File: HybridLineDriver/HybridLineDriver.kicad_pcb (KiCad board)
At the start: 2 copper layers, 100 x 100 mm, 34 parts, among them J1 XLR3, J2 Conn_01x03, J3 Conn_01x02, U1 OPA1679

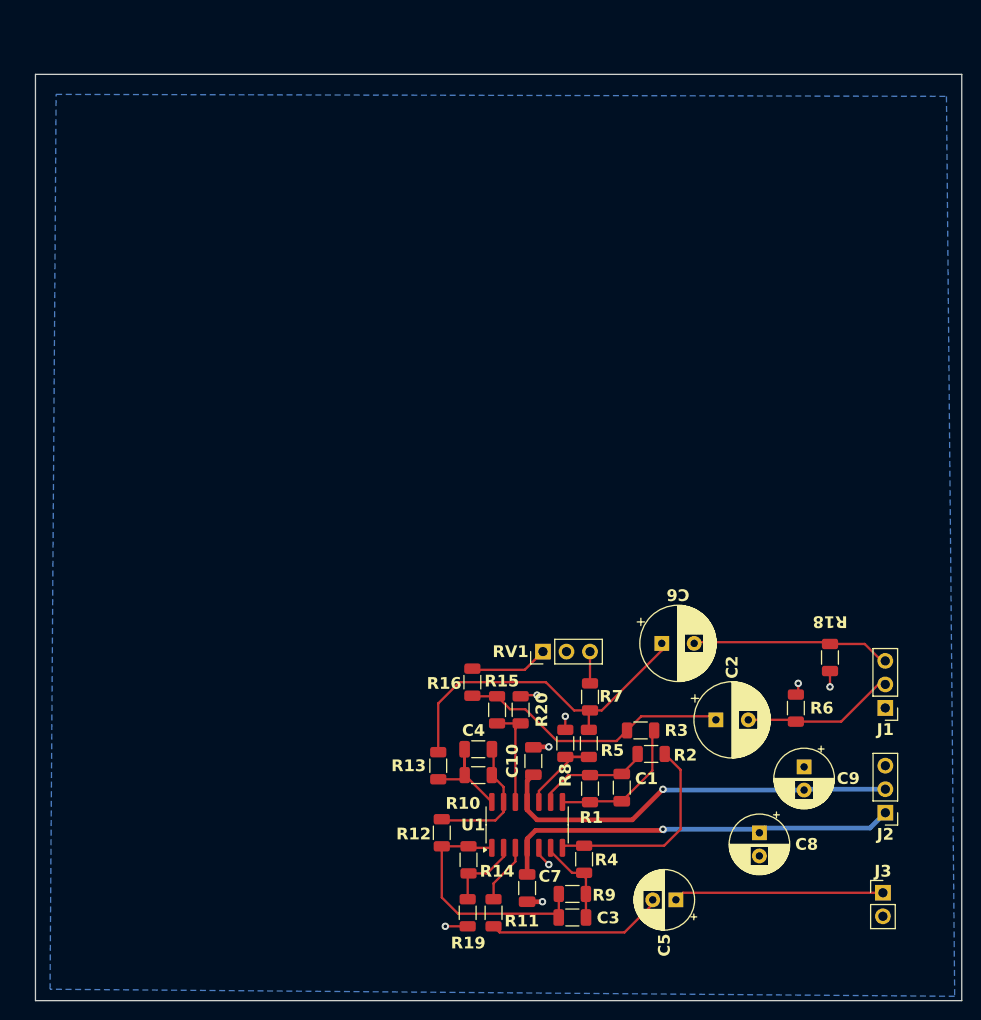
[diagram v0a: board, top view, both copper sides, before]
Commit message: pcb cleanup
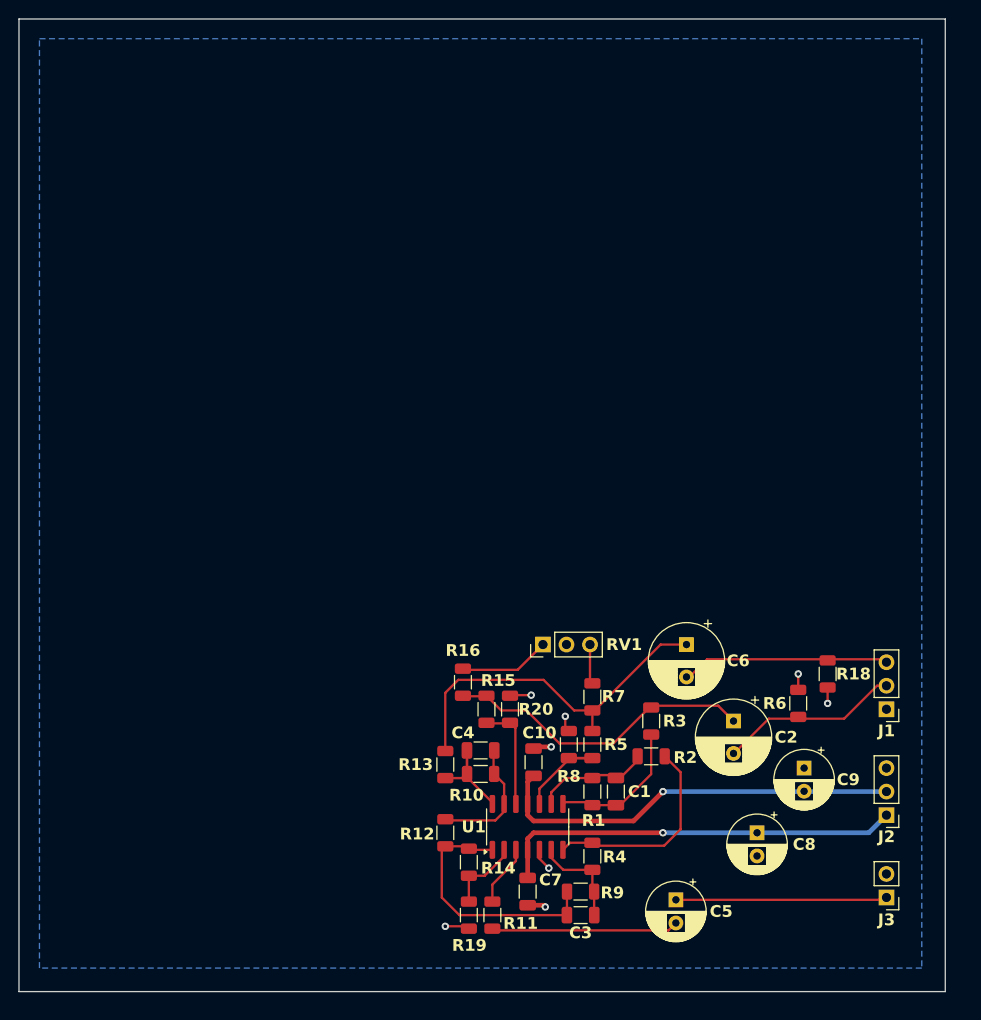
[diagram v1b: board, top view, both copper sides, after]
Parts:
- moved C6 2.67 mm to (113.0, 93.3), turned to -90 degrees
- moved C2 1.91 mm to (118.1, 101.6), turned to -90 degrees
- moved R18 1.80 mm to (128.3, 96.5)
- moved R3 1.53 mm to (109.2, 101.6), turned to 90 degrees
- moved R15 1.14 mm to (91.4, 100.3)
- moved R20 1.14 mm to (94.0, 100.3)
- moved R16 1.02 mm to (88.9, 97.4)
- moved R4 0.94 mm to (102.9, 116.2)
- moved R9 0.92 mm to (101.6, 120.0)
- moved C3 0.92 mm to (101.6, 122.6)
- moved R13 0.77 mm to (87.0, 106.3)
- moved C1 0.77 mm to (105.4, 109.2)
- moved RV1 0.76 mm to (97.5, 93.3)
- moved J3 0.64 mm to (134.6, 120.7), turned to 180 degrees
- moved R6 0.57 mm to (125.1, 99.7)
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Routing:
- net Net-(C2-Pad1): track 29.6 -> 34.5 mm
- net Net-(C2-Pad2): track 16.5 -> 20.3 mm
- net Net-(C6-Pad1): track 37.2 -> 40.3 mm
- net GND: track 14.3 -> 16.2 mm
- net Net-(R16-Pad2): track 8.49 -> 9.82 mm
- net Net-(U1B--): track 9.86 -> 11.0 mm
- net Net-(C6-Pad2): track 21.5 -> 22.6 mm
- net Net-(C5-Pad2): track 19.2 -> 20.2 mm
- net Net-(C3-Pad1): track 27.1 -> 28.1 mm
- net Net-(R7-Pad1): track 3.42 -> 4.29 mm
- net Net-(C4-Pad2): track 12.8 -> 11.9 mm
- net +15V: track 44.8 -> 44.0 mm
- net Net-(U1D--): track 14.6 -> 13.9 mm
- net Net-(U1C-+): track 10.6 -> 11.3 mm
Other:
- board size 100 x 100 mm -> 100 x 105 mm
